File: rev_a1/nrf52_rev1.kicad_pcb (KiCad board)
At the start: 2 copper layers, 48.3 x 48.3 mm, 31 parts, among them P1 CONN_01X18, P2 CONN_01X18, P3 USB_OTG, U1 nRF52832, U2 CP2102, U3 LT1129CST-3.3, Y1 32K, Y2 32M

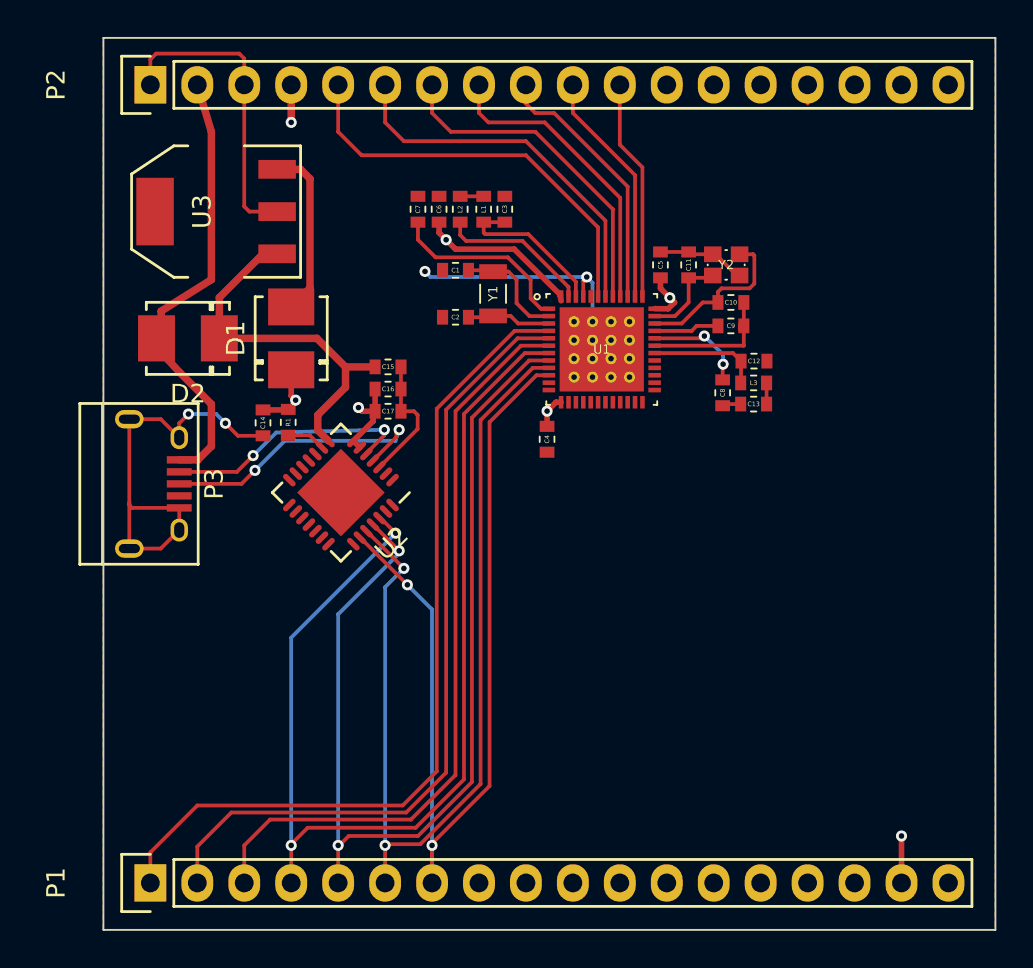
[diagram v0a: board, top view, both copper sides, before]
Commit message: wip
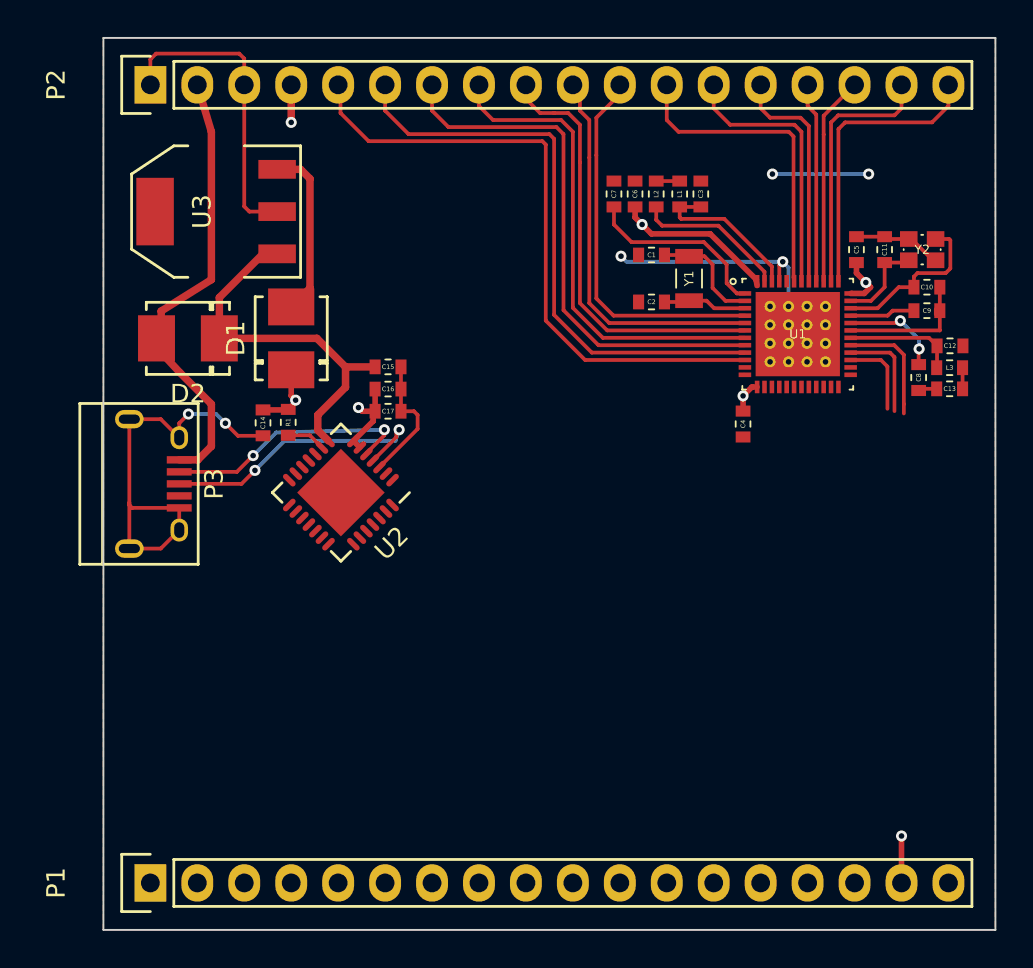
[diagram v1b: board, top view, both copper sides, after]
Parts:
- moved C10 10.6 mm to (70.0, 38.9)
- moved C11 10.6 mm to (67.7, 36.9)
- moved C12 10.6 mm to (71.2, 42.1)
- moved C3 10.6 mm to (57.7, 33.8)
- moved C4 10.6 mm to (60.0, 46.3)
- moved C5 10.6 mm to (66.1, 36.9)
- moved C6 10.6 mm to (54.2, 33.8)
- moved C7 10.6 mm to (53.0, 33.8)
- moved C9 10.6 mm to (70.0, 40.2)
- moved L1 10.6 mm to (56.6, 33.8)
- moved L2 10.6 mm to (55.3, 33.8)
- moved U1 10.6 mm to (63.0, 41.4)
- moved Y1 10.6 mm to (57.1, 38.4)
- moved C1 10.6 mm to (55.1, 37.1)
- moved C13 10.6 mm to (71.2, 44.4)
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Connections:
- P1 pad 1: P0.02 -> P0.11
- P1 pad 10: P0.13 -> P0.20
- P1 pad 11: P0.14 -> P0.21
- P1 pad 12: P0.15 -> SWDCLK
- P1 pad 13: P0.16 -> SWDIO
- P1 pad 14: P0.17 -> P0.22
- P1 pad 15: P0.18 -> P0.23
- P1 pad 16: P0.19 -> P0.24
- P1 pad 2: P0.03 -> P0.12
- P1 pad 3: P0.04 -> P0.13
- P1 pad 4: P0.05 -> P0.14
- P1 pad 5: P0.06 -> P0.15
- P1 pad 6: P0.07 -> P0.16
- P1 pad 7: P0.08 -> P0.17
- P1 pad 8: P0.11 -> P0.18
- P1 pad 9: P0.12 -> P0.19
- P2 pad 10: P0.26 -> P0.03
- P2 pad 11: P0.25 -> P0.02
- P2 pad 12: P0.24 -> P0.31
- P2 pad 13: P0.23 -> P0.30
- P2 pad 14: P0.22 -> P0.29
- P2 pad 15: SWDIO -> P0.28
- P2 pad 16: SWDCLK -> P0.27
- P2 pad 17: P0.21 -> P0.26
- P2 pad 18: P0.20 -> P0.25
- P2 pad 5: P0.31 -> P0.08
- P2 pad 6: P0.30 -> P0.07
- P2 pad 7: P0.29 -> P0.06
- P2 pad 8: P0.28 -> P0.05
- P2 pad 9: P0.27 -> P0.04
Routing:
- net P0.05: track 60.0 -> 26.4 mm, vias 2 -> 0
- net P0.06: track 55.2 -> 29.2 mm, vias 2 -> 0
- net P0.02: track 46.4 -> 20.5 mm
- net P0.03: track 44.8 -> 21.0 mm
- net P0.07: track 51.4 -> 31.9 mm, vias 2 -> 0
- net P0.04: track 41.2 -> 23.5 mm
- net P0.08: track 50.8 -> 35.4 mm, vias 2 -> 0
- net P0.31: track 23.2 -> 17.0 mm
- net P0.24: track 0.00 -> 6.27 mm
- net P0.30: track 20.3 -> 14.6 mm
- net P0.29: track 18.2 -> 12.7 mm
- net P0.23: track 0.00 -> 5.39 mm
- net (no net): track 0.00 -> 5.21 mm, vias 0 -> 2
- net P0.22: track 0.00 -> 4.42 mm
- net P0.28: track 16.4 -> 12.5 mm
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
